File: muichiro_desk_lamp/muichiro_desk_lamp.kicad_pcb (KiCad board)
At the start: 2 copper layers, 102.6 x 123.6 mm, 7 parts, among them J1 Conn_01x03_Pin, U1 ESP32-C3-DevKitM-1

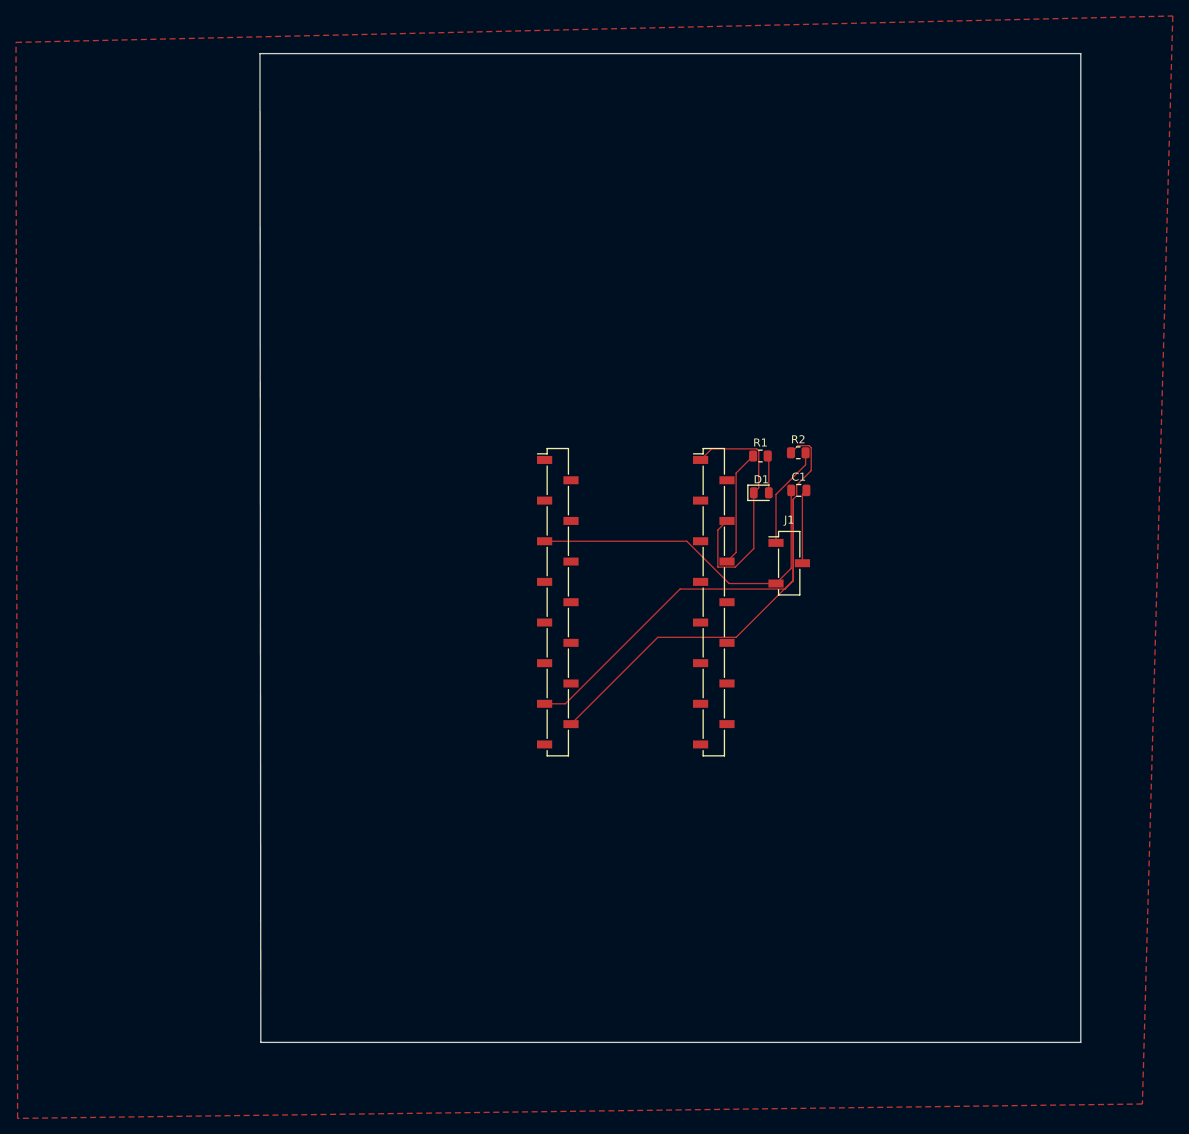
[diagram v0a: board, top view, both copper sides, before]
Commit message: updated muichiro_desk_lamp
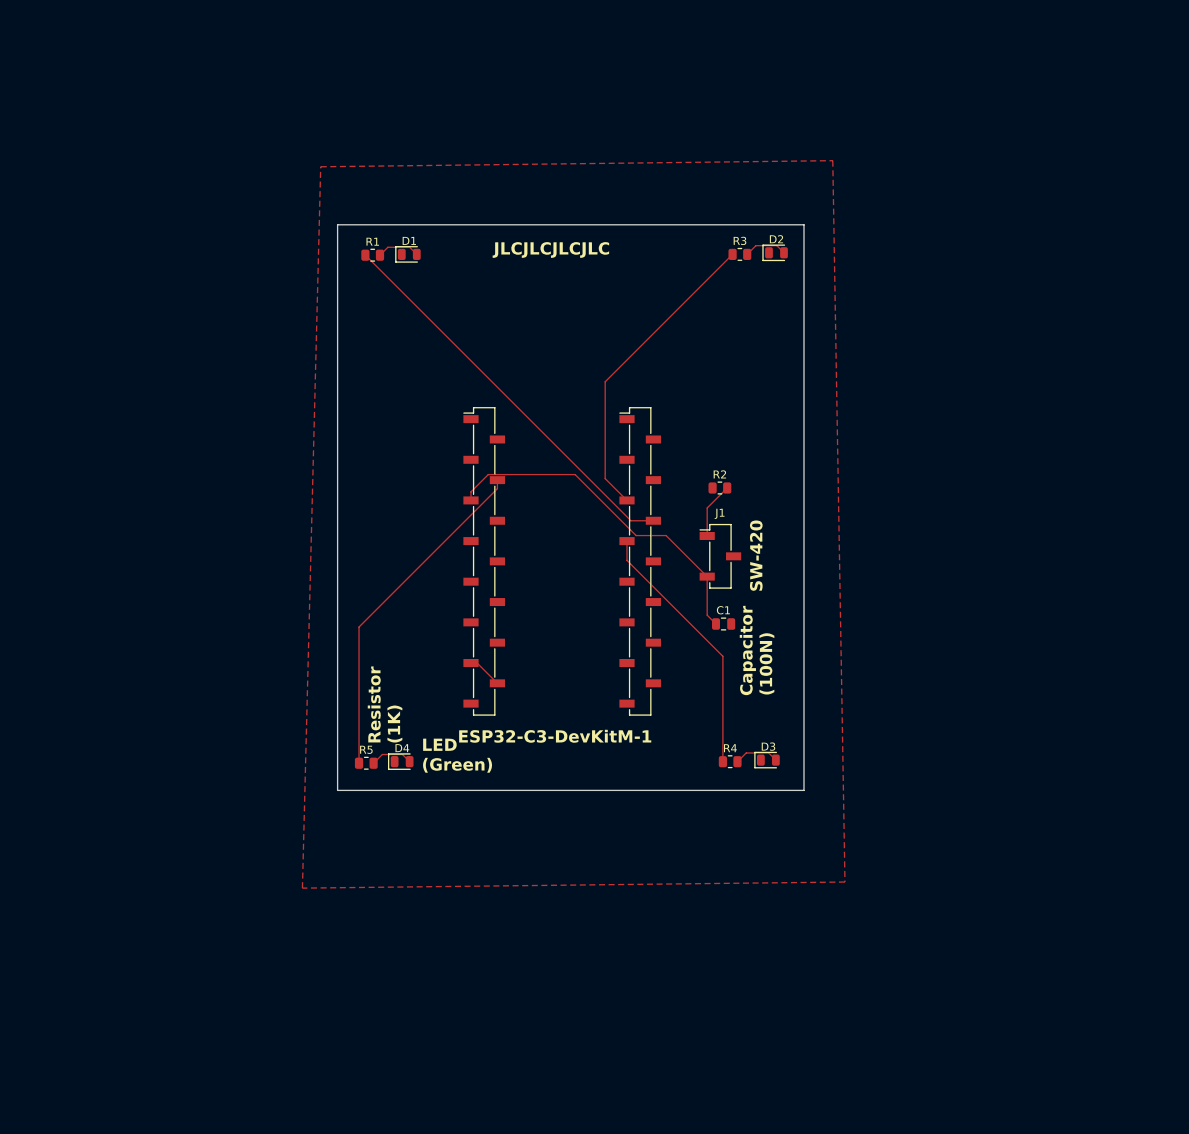
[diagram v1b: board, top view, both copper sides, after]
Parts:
- added D2: LED, LED_SMD:LED_0805_2012Metric, F.Cu at (192.9, 48.6)
- added D3: LED, LED_SMD:LED_0805_2012Metric, F.Cu at (191.8, 112.0)
- added D4: LED, LED_SMD:LED_0805_2012Metric, F.Cu at (146.1, 112.2)
- added R3: 1K, Resistor_SMD:R_0805_2012Metric, F.Cu at (188.3, 48.8)
- added R4: 1K, Resistor_SMD:R_0805_2012Metric, F.Cu at (187.1, 112.2)
- added R5: 1K, Resistor_SMD:R_0805_2012Metric, F.Cu at (141.6, 112.4)
- moved R1 54.6 mm to (142.4, 48.9)
- moved D1 53.1 mm to (147.0, 48.8)
- moved C1 19.2 mm to (186.2, 95.0)
- moved G*** 13.7 mm to (167.1, 80.5)
- moved R2 10.7 mm to (185.8, 78.0)
- moved U1 10.5 mm to (166.7, 107.0)
- moved J1 8.64 mm to (185.8, 86.5)
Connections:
- R2 pad 1: +5V -> +3V3
- U1 pad 20: unconnected-(U1-IO4-Pad20) -> Net-(U1-IO4)
- U1 pad 22: unconnected-(U1-IO6-Pad22) -> Net-(U1-IO6)
- U1 pad 4: unconnected-(U1-IO2-Pad4) -> Net-(U1-IO2)
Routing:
- net +5V: track 103.4 -> 4.35 mm
- net Net-(U1-IO2): track 0.00 -> 42.6 mm
- net GND: track 41.4 -> 0.00 mm
- net Net-(U1-IO4): track 0.00 -> 38.5 mm
- net Net-(U1-IO5): track 14.5 -> 49.7 mm
- net Net-(U1-IO6): track 0.00 -> 32.5 mm
- net Net-(J1-Pin_1): track 12.8 -> 7.04 mm
- net Net-(D3-A): track 0.00 -> 5.62 mm
- net Net-(D2-A): track 0.00 -> 5.42 mm
- net Net-(D4-A): track 0.00 -> 5.32 mm
- net Net-(D1-A): track 4.65 -> 5.38 mm
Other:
- board size 102.6 x 123.6 mm -> 58.3 x 70.7 mm
- board text added: "Capacitor (100N)"
- board text added: "ESP32-C3-DevKitM-1"
- board text added: "JLCJLCJLCJLC"
- board text added: "LED (Green)"
- board text added: "Resistor (1K)"
- board text added: "SW-420"
